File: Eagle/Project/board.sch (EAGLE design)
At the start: 18 parts, among them IC1 ATTINY402-SSF, X1 PAD-1.27X2.54, X2 PAD-1.27X2.54, X3 PAD-1.27X2.54

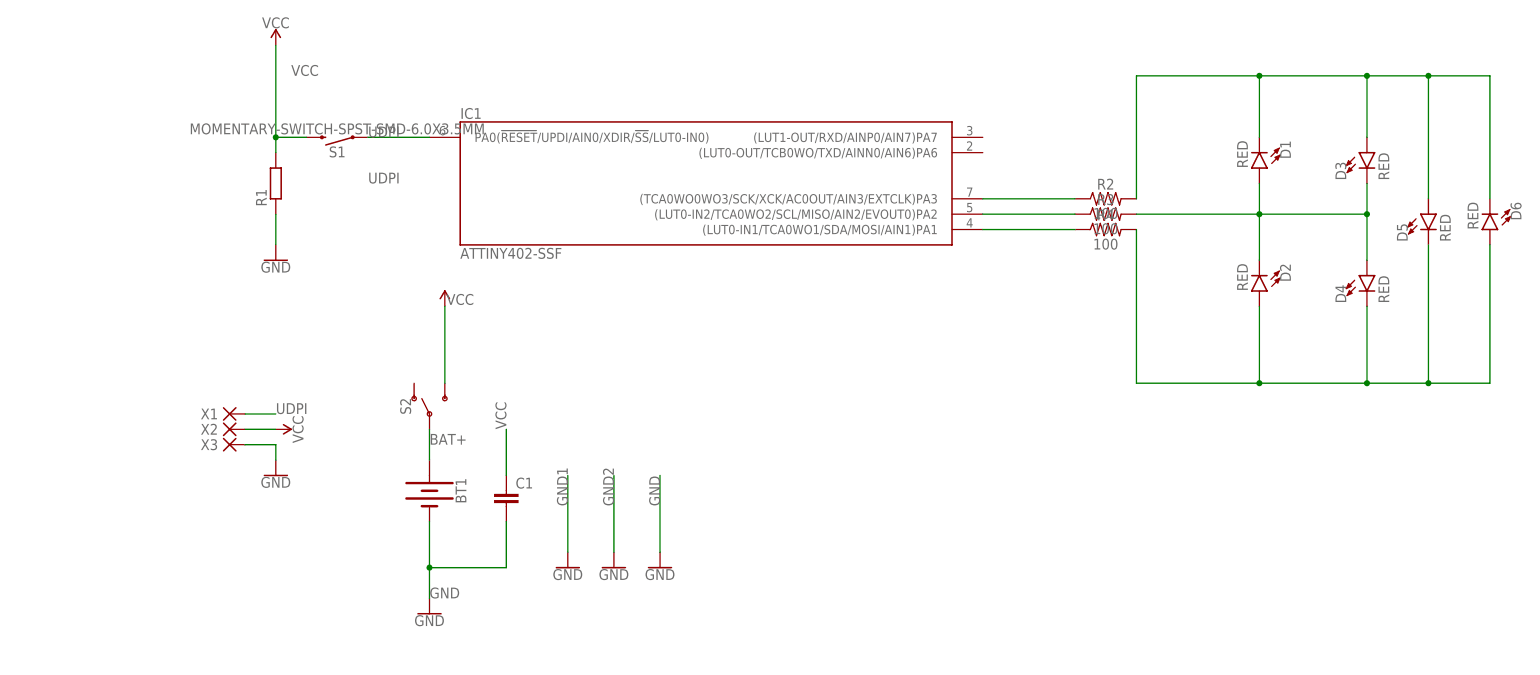
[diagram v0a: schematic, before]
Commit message: Updated project
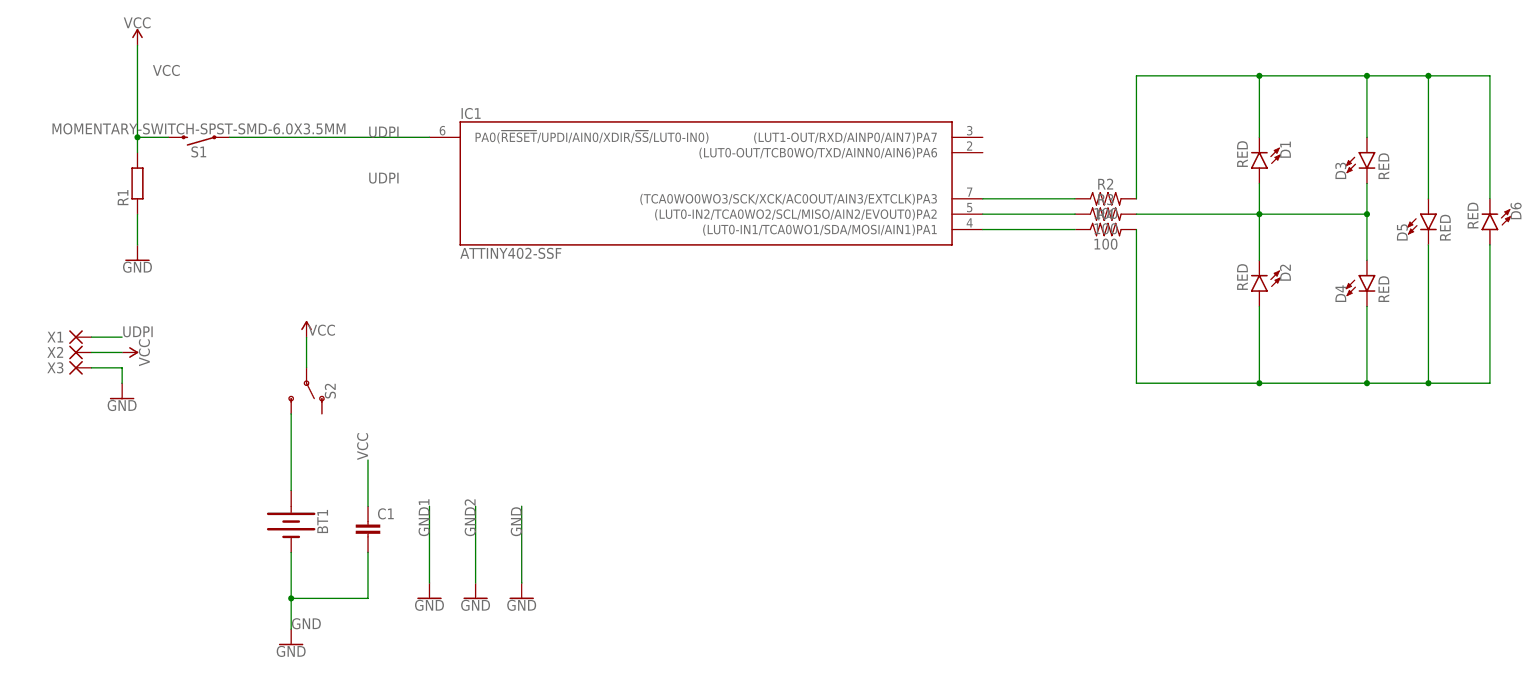
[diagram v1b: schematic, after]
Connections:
- removed net BAT+: BT1.+, S2.P
- new net N$6: BT1.+, S2.S
- net VCC: now also S2.P; no longer S2.S
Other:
- moved on the sheet: BT1, C1, R1, S1, S2, X1, X2, X3
